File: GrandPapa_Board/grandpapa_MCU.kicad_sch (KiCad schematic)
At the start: 1 part, among them U1 DSPIC33EP512GP502

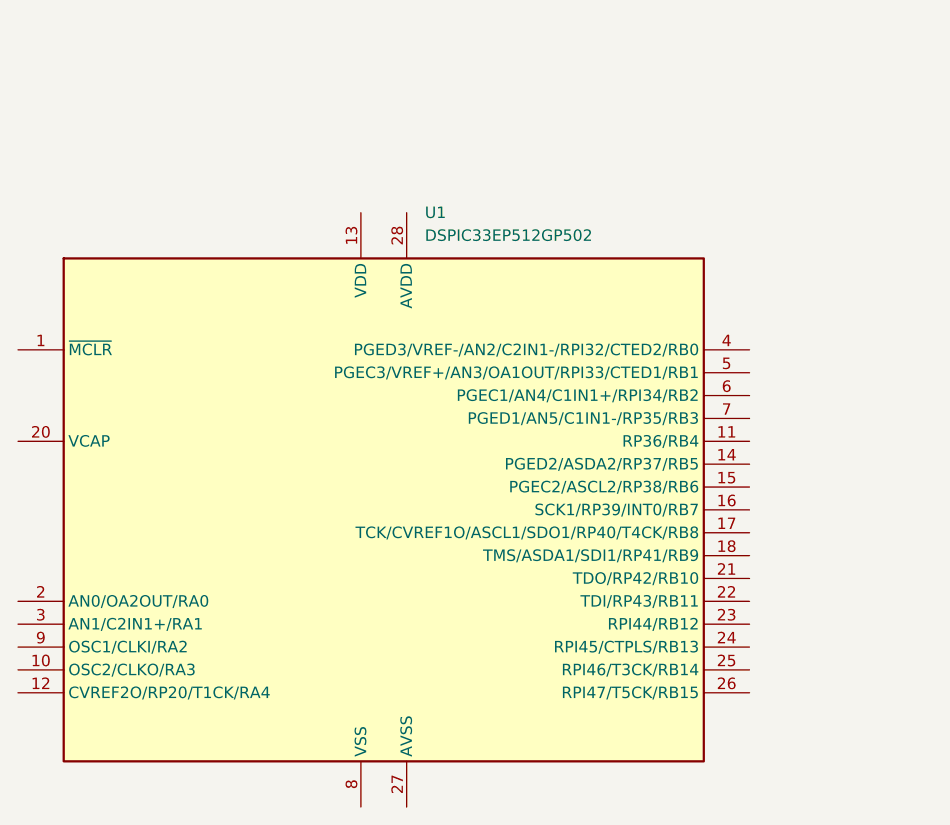
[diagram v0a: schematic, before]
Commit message: Shameless papa copying pt 1
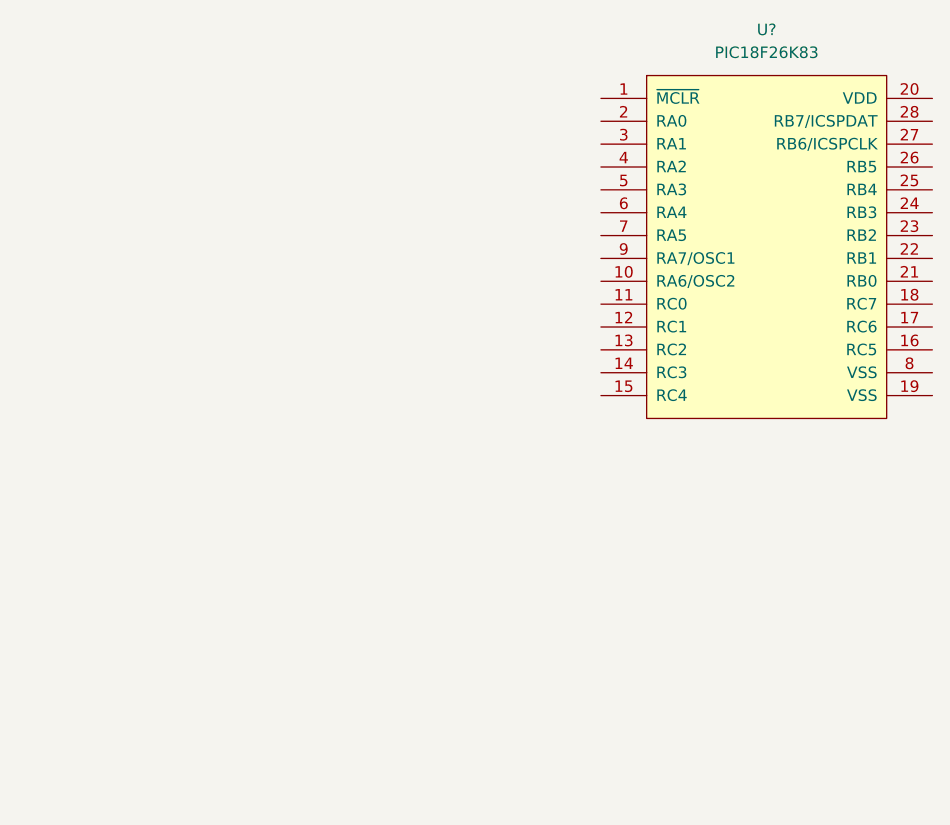
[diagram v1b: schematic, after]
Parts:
- removed U1: DSPIC33EP512GP502, Package_DIP:DIP-28_W7.62mm, symbol CANHW:DSPIC33EP512GP502
- added U?: PIC18F26K83, symbol CANHW:PIC18F26K83
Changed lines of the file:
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@@
 (kicad_sch (version 20211123) (generator eeschema)
   (paper "A4")
-  (symbol (lib_id "CANHW:DSPIC33EP512GP502") (at 93.98 128.27 0) (unit 1)
+  (symbol (lib_id "CANHW:PIC18F26K83") (at 137.16 99.06 0) (unit 1)
     (in_bom yes) (on_board yes) (fields_autoplaced)
-    (property "Reference" "U1" (id 0) (at 98.5394 95.25 0)
-      (effects (font (size 1.27 1.27)) (justify left))
-    )
-    (property "Value" "DSPIC33EP512GP502" (id 1) (at 98.5394 97.79 0)
-      (effects (font (size 1.27 1.27)) (justify left))
-    )
-    (property "Footprint" "Package_DIP:DIP-28_W7.62mm" (id 2) (at 93.98 128.27 0)
+    (property "Reference" "U?" (id 0) (at 136.525 74.93 0))
+    (property "Value" "PIC18F26K83" (id 1) (at 136.525 77.47 0))
+    (property "Footprint" "" (id 2) (at 148.59 99.06 0)
       (effects (font (size 1.27 1.27)) hide)
     )
-    (property "Datasheet" "" (id 3) (at 93.98 128.27 0)
+    (property "Datasheet" "http://ww1.microchip.com/downloads/en/DeviceDoc/40001943A.pdf" (id 3) (at 148.59 99.06 0)
       (effects (font (size 1.27 1.27)) hide)
     )
